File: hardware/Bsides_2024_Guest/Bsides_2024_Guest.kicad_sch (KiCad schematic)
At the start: 39 parts, among them J1 Conn_02x03_Odd_Even, J2 Battery, J3 Battery, J4 OLED, P1 USB_C_Plug_USB2.0, Q1 DMG3415U-7, SW1 ON, SW2 RESET, SW3 BOOT, SW4 RESET, SW6 RESET, U1 ESP32-C6-WROOM-1U-N4, U2 AP2112K-3.3

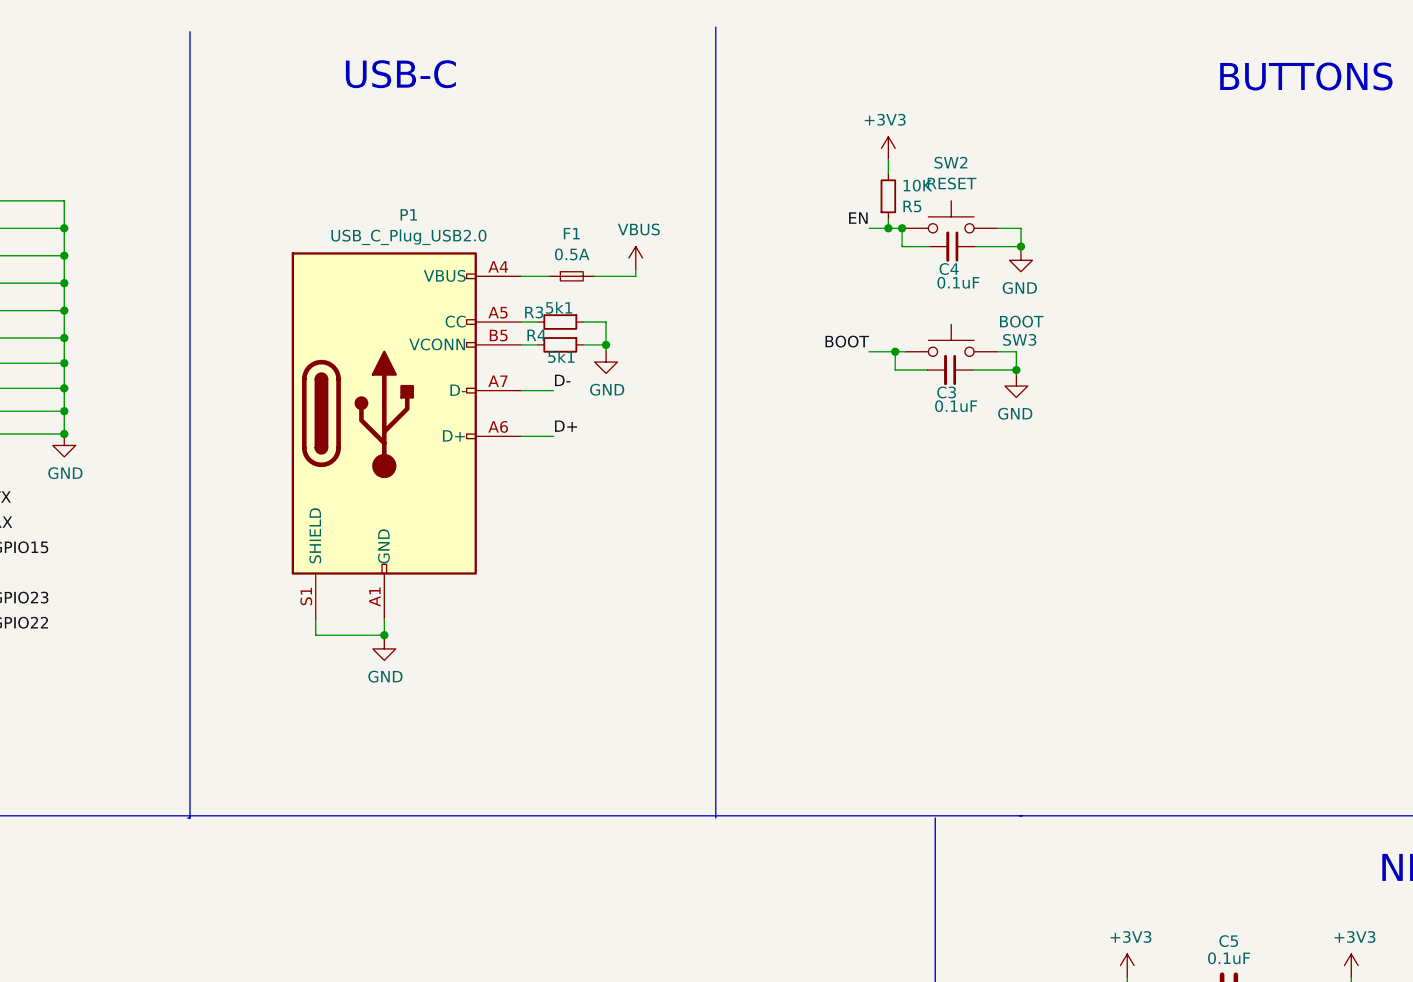
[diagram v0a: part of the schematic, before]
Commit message: feat(Hw): Shitty Addon PCB added
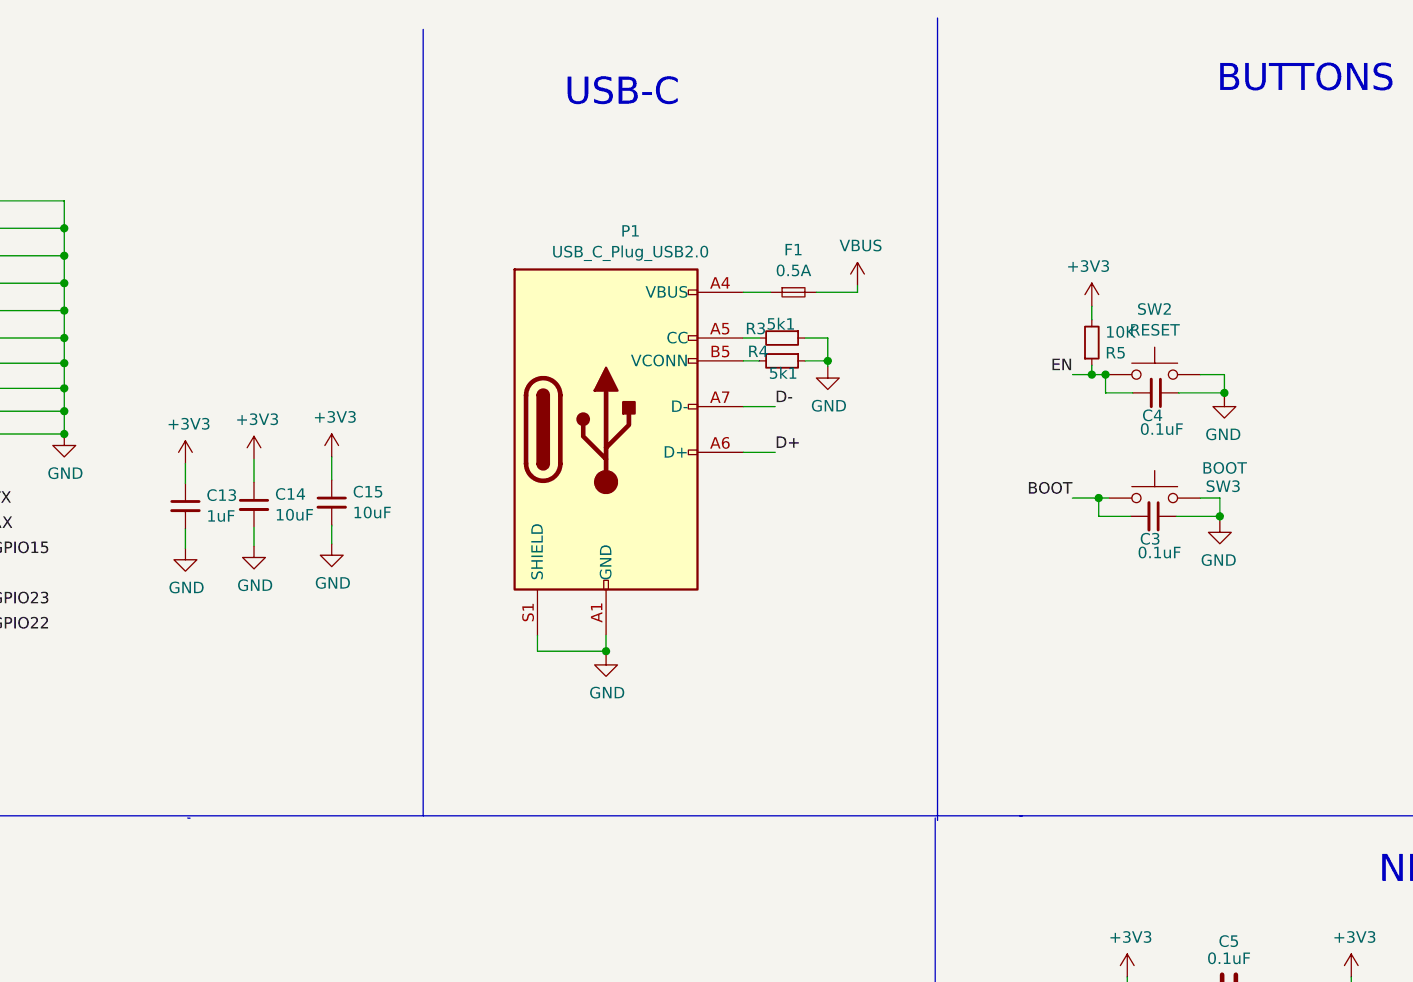
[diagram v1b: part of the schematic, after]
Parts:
- added C13: 1uF, Capacitor_SMD:C_0603_1608Metric, symbol Device:C_Small
- added C14, C15: 10uF, Capacitor_SMD:C_0603_1608Metric, symbol Device:C_Small
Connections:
- net +3V3: now also C13.1, C14.1, C15.1
- net GND: now also C13.2, C14.2, C15.2
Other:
- moved on the sheet: C3, C4, F1, P1, R3, R4, R5, SW2, SW3
